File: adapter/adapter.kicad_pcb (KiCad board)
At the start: 2 copper layers, 41.8 x 50.8 mm, 30 parts, among them J1 Serial, J2 Battery charge, J3 Ribbon, J4 Ribbon, J5 RGB, SW1 SW_SPST, SW3 SW_SPDT, U1 Dual MCU: RP2040 + nice!nano, U2 AP1603WG-7, U3 USBLC6-2P6

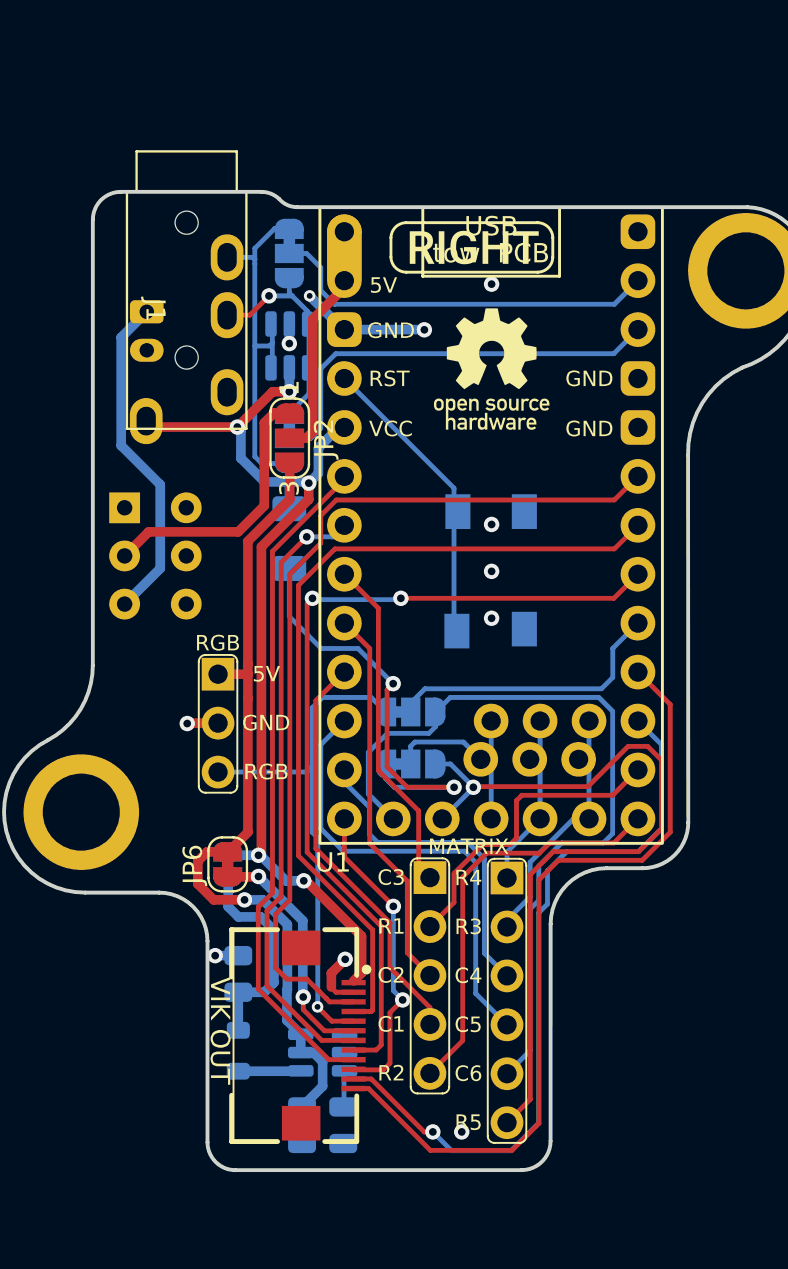
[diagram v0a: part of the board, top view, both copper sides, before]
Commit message: WIP - RECORD POSITIONS AND REVERT
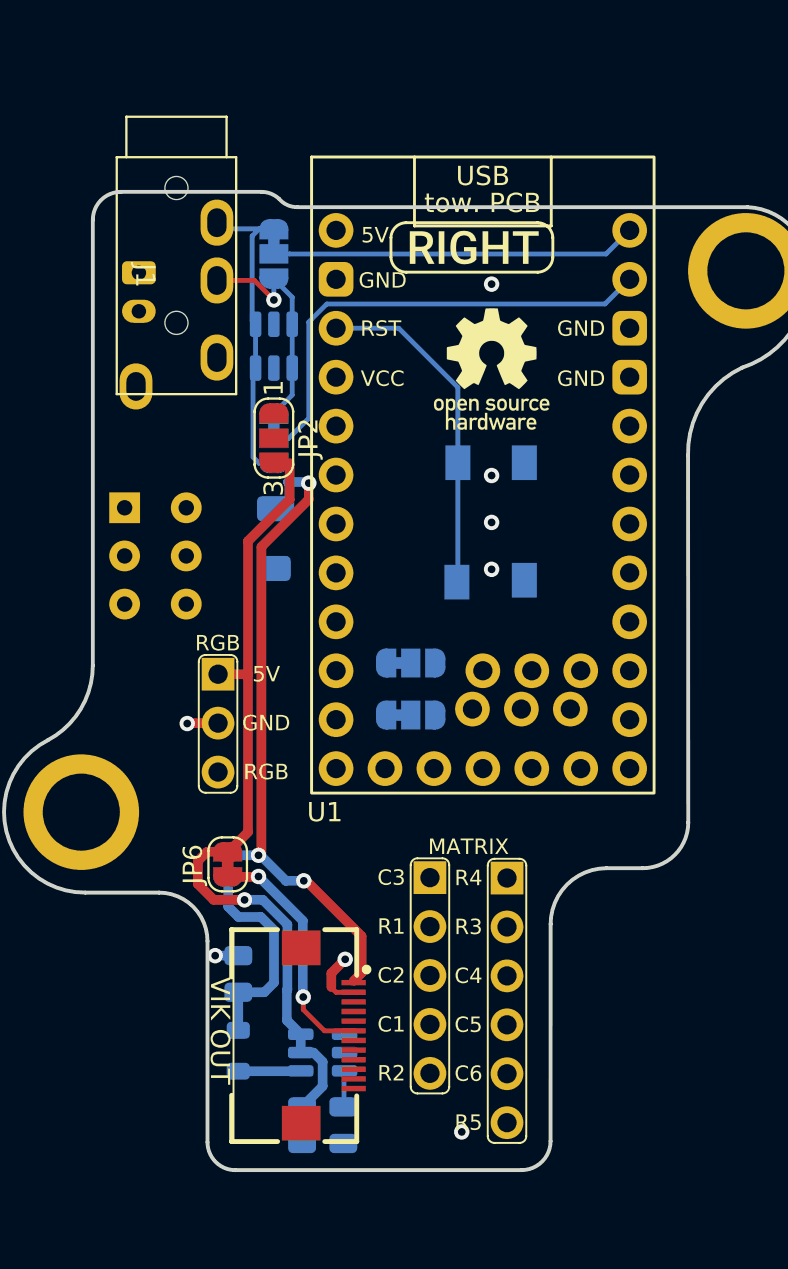
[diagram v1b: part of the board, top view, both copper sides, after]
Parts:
- moved U1 2.65 mm to (137.7, 81.9)
- moved JP3 2.54 mm to (134.0, 94.4)
- moved JP7 2.54 mm to (134.0, 91.7)
- moved SW1 2.54 mm to (138.2, 84.4)
- moved kibuzzard-61F01C84 2.54 mm to (142.1, 84.3)
- moved J2 2.07 mm to (119.9, 71.4)
- moved J1 1.88 mm to (121.8, 71.5)
- moved JP2 0.82 mm to (126.9, 80.0)
- moved JP1 0.80 mm to (126.9, 70.4)
- moved U3 0.80 mm to (126.9, 75.2)
- moved JP5 0.80 mm to (126.9, 80.0)
- moved R1 0.80 mm to (126.9, 85.2)
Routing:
- net SDA_L: track 46.5 -> 0.00 mm
- net MOSI_L: track 43.9 -> 0.00 mm, vias 2 -> 0
- net SCL_L: track 43.6 -> 0.00 mm
- net SCLK_L: track 41.0 -> 0.00 mm
- net col6_l: track 40.9 -> 0.00 mm
- net row5_l: track 40.4 -> 0.00 mm, vias 1 -> 0
- net MISO_L: track 37.9 -> 0.00 mm, vias 1 -> 0
- net GPIO_2_L: track 34.8 -> 0.00 mm
- net GPIO_1_L: track 32.0 -> 0.00 mm, vias 1 -> 0
- net RGB_L: track 27.1 -> 0.00 mm, vias 1 -> 0
- net col5_l: track 24.0 -> 0.00 mm
- net Net-(JP3-A): track 22.2 -> 0.00 mm, vias 2 -> 0
- net col1_l: track 21.4 -> 0.00 mm
- net row2_l: track 21.2 -> 0.00 mm
- net col2_l: track 20.1 -> 0.00 mm
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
